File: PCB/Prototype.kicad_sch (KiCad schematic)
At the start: 7 parts, among them SW5 SW_Push, SW6 SW_Push, SW7 SW_Push, SW8 SW_Push, U1 XIAO-RP2040-DIP

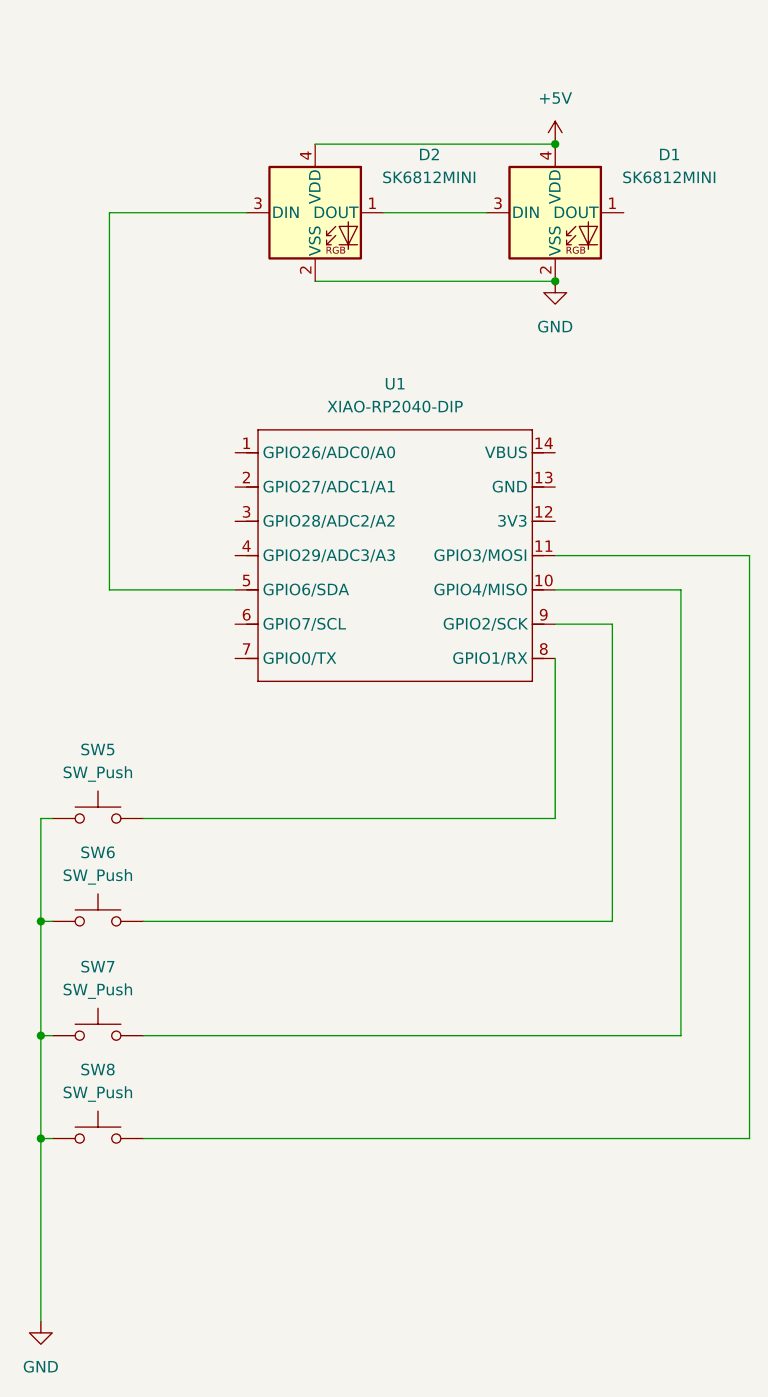
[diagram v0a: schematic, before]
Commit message: Initial commit!!
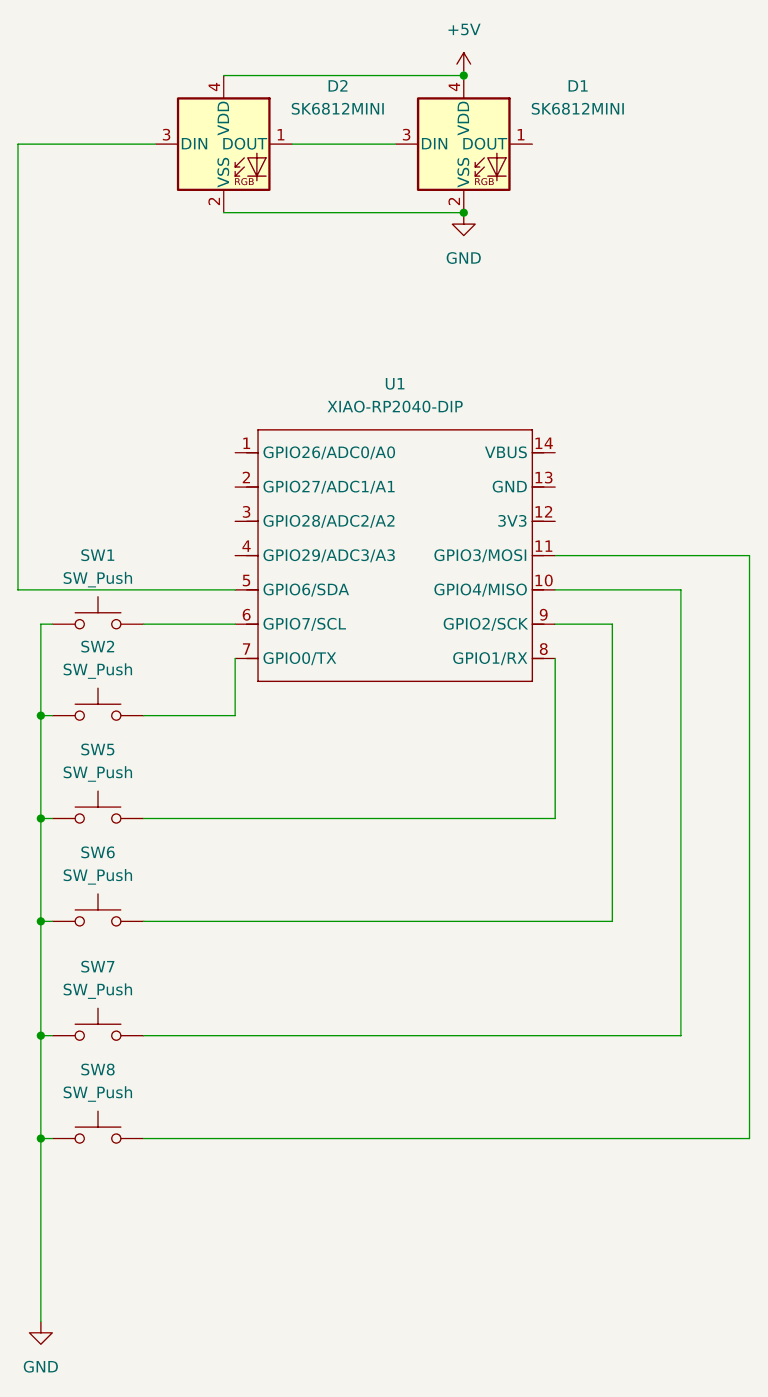
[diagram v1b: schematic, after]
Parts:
- added SW1, SW2: SW_Push, Button_Switch_Keyboard:SW_Cherry_MX_1.00u_PCB, symbol Switch:SW_Push
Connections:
- net GND: now also SW1.1, SW2.1
- net at U1.6 (GPIO7/SCL): now also SW1.2
- net at U1.7 (GPIO0/TX): now also SW2.2
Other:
- moved on the sheet: D1, D2
